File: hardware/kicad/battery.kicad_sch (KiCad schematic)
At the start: 1 part, among them J1 JST-2PH

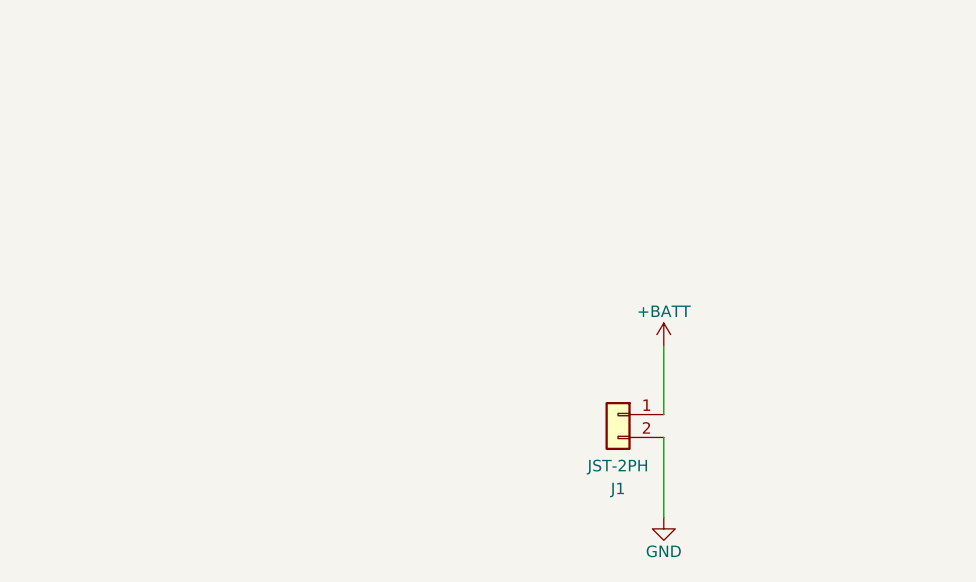
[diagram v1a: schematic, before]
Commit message: wip: revision 2
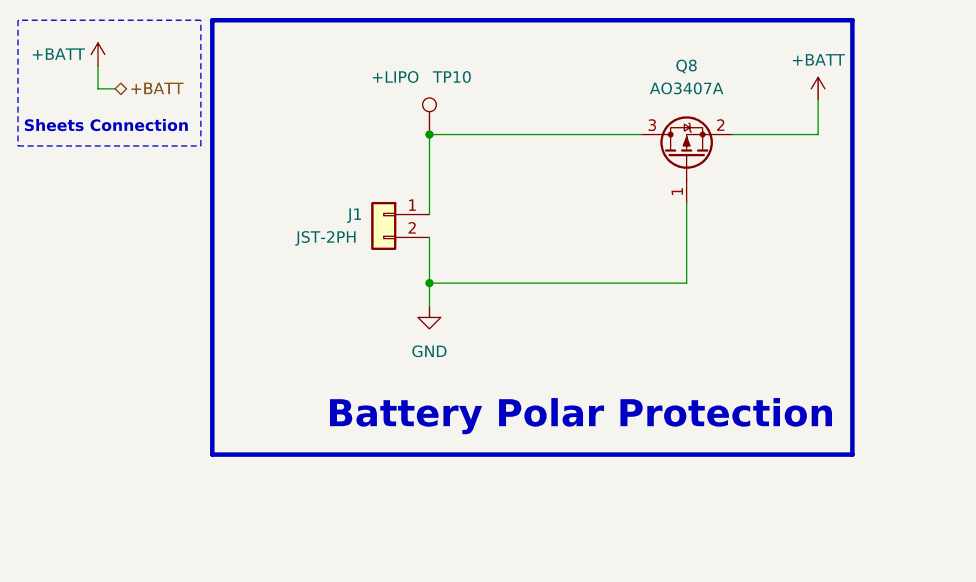
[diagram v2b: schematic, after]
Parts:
- added Q8: AO3407A, Package_TO_SOT_SMD:SOT-23, symbol Device:Q_PMOS_GSD
- added TP10: +LIPO, TestPoint:TestPoint_Pad_D1.0mm, symbol Connector:TestPoint
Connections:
- net +BATT: now also Q8.2 (S); no longer J1.1 (Pin_1)
- net GND: now also Q8.1 (G)
- new net: J1.1 (Pin_1), Q8.3 (D), TP10.1
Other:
- note added: "Battery Polar Protection"
- note added: "Sheets Connection"
- moved on the sheet: J1

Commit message: wip: revision 2
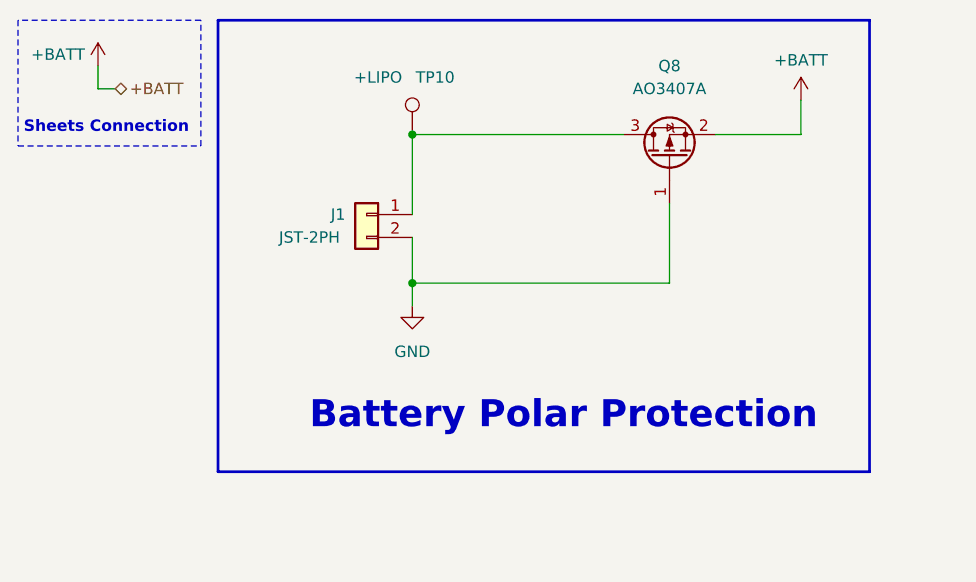
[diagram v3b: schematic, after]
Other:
- moved on the sheet: J1, Q8, TP10
